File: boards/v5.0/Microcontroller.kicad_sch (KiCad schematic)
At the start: 10 parts, among them P1 Pin Socket 2.54mm 02x22, P2 Pin Socket 2.54mm 01x22, U2 TXS0108EPW

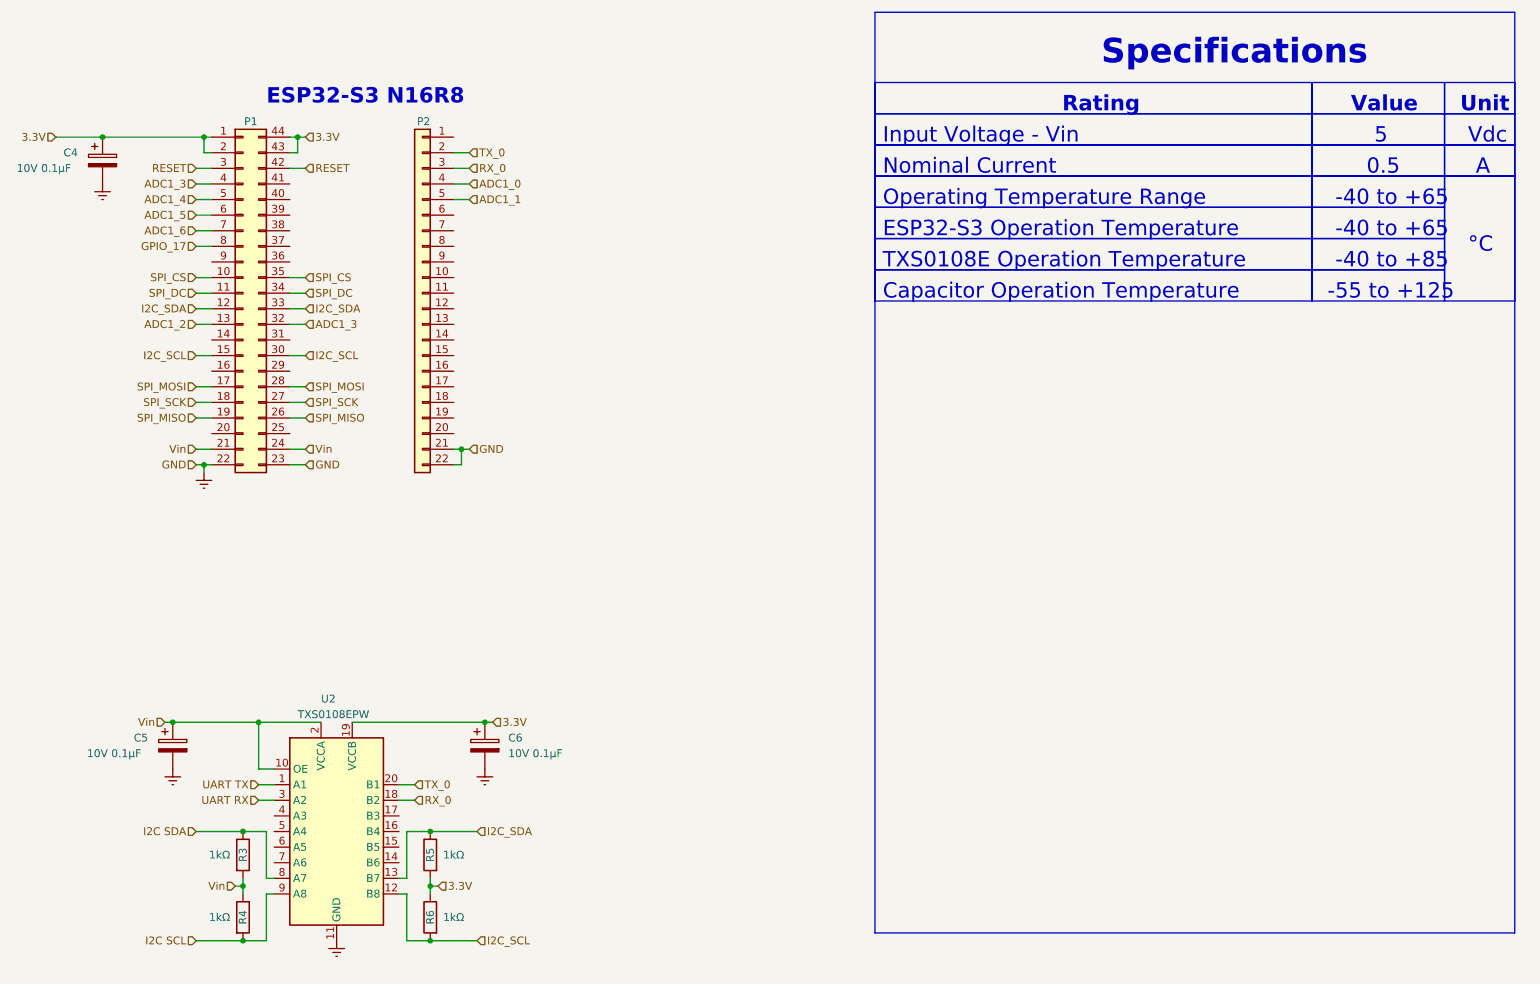
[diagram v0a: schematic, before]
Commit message: Update board v5.0 docs
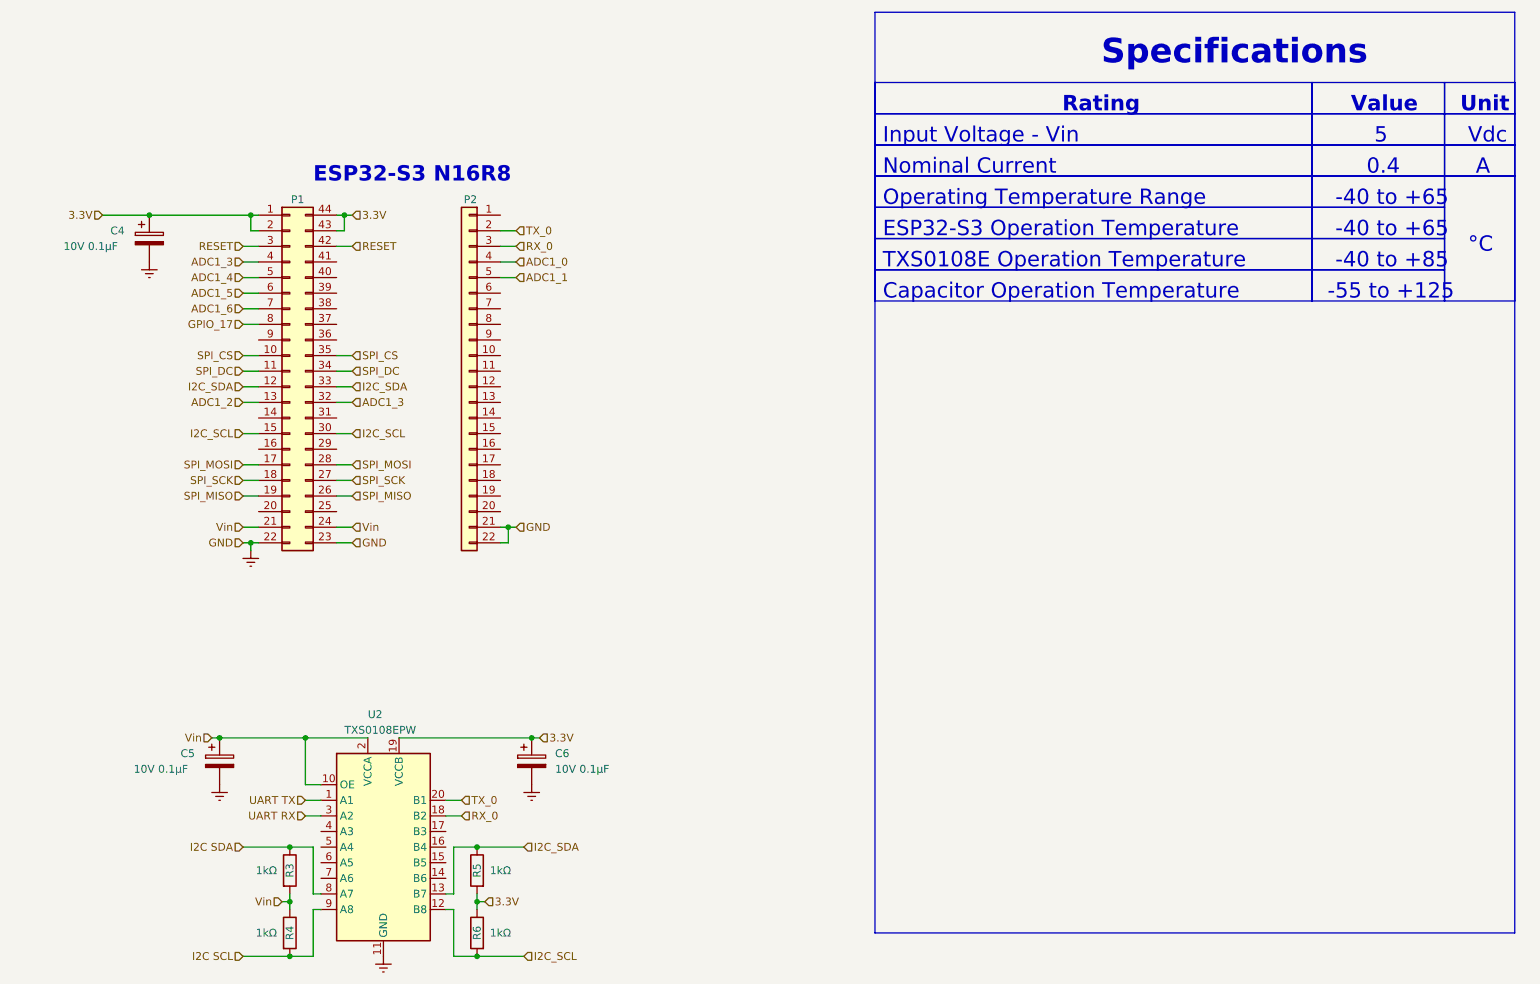
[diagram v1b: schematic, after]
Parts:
- P1: footprint (none) -> Connector_PinSocket_2.54mm:PinSocket_2x22_P2.54mm_Vertical
- P2: footprint (none) -> Connector_PinSocket_2.54mm:PinSocket_1x22_P2.54mm_Vertical
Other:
- note added: "0.4"
- note removed: "0.5"
- company: Power Vision -> Lucas Rayan Guerra da Silva
- moved on the sheet: C4, C5, C6, P1, P2, R3, R4, R5, R6, U2
